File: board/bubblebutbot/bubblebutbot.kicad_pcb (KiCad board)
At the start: 2 copper layers, 94 x 32.5 mm, 55 parts, among them J1 JST XH, J10 JST XH, J11 JST XH, J13 JST XH, J2 USB_C_Receptacle, J3 Conn_01x03_Socket, J4 Conn_01x03_Socket, J5 Conn_01x03_Socket, J6 Conn_01x03_Socket, J7 Conn_01x03_Socket, J8 Conn_01x03_Socket, J9 JST XH, Q1 FDN336P, SW1 SW_Push, SW2 SW_Push, U1 DRV8833PWP, U2 ESP32-S3-WROOM-1, U3 AP2112K-3.3, U4 LIS3DH

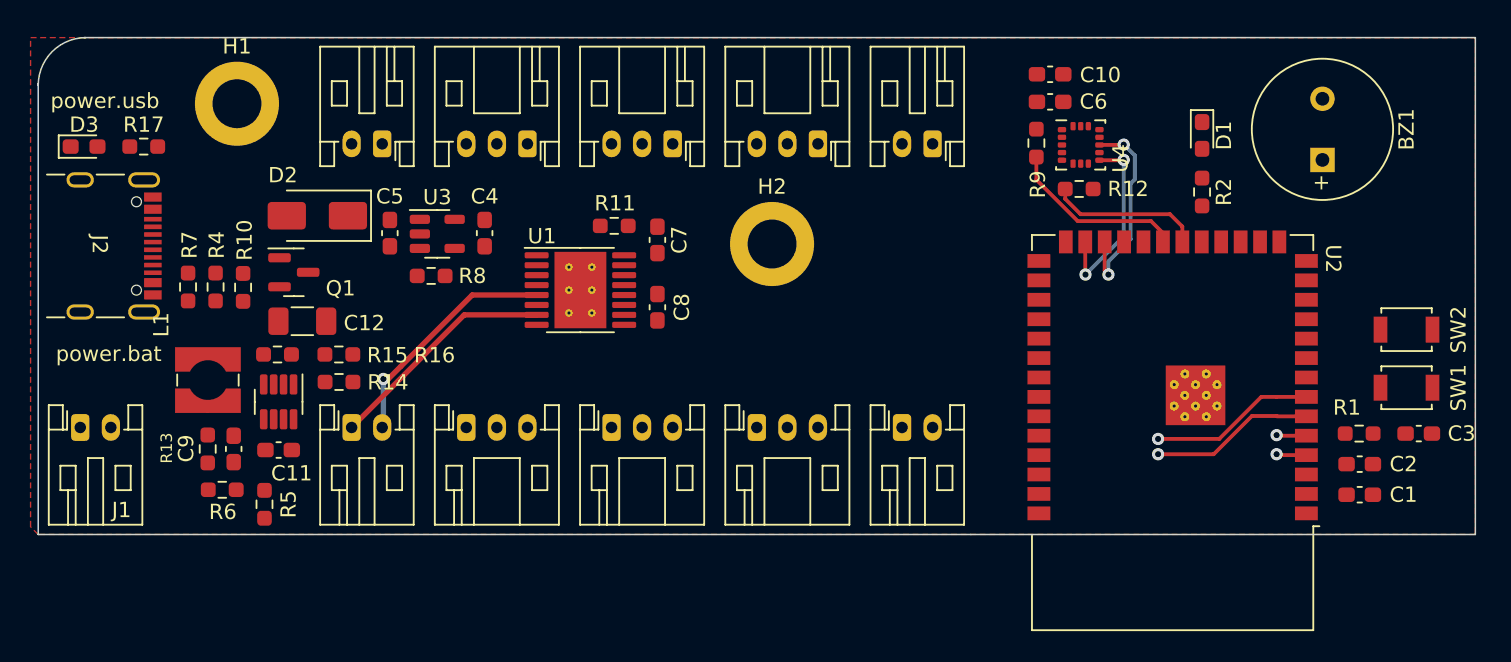
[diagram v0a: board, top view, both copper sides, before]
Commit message: pcb done!
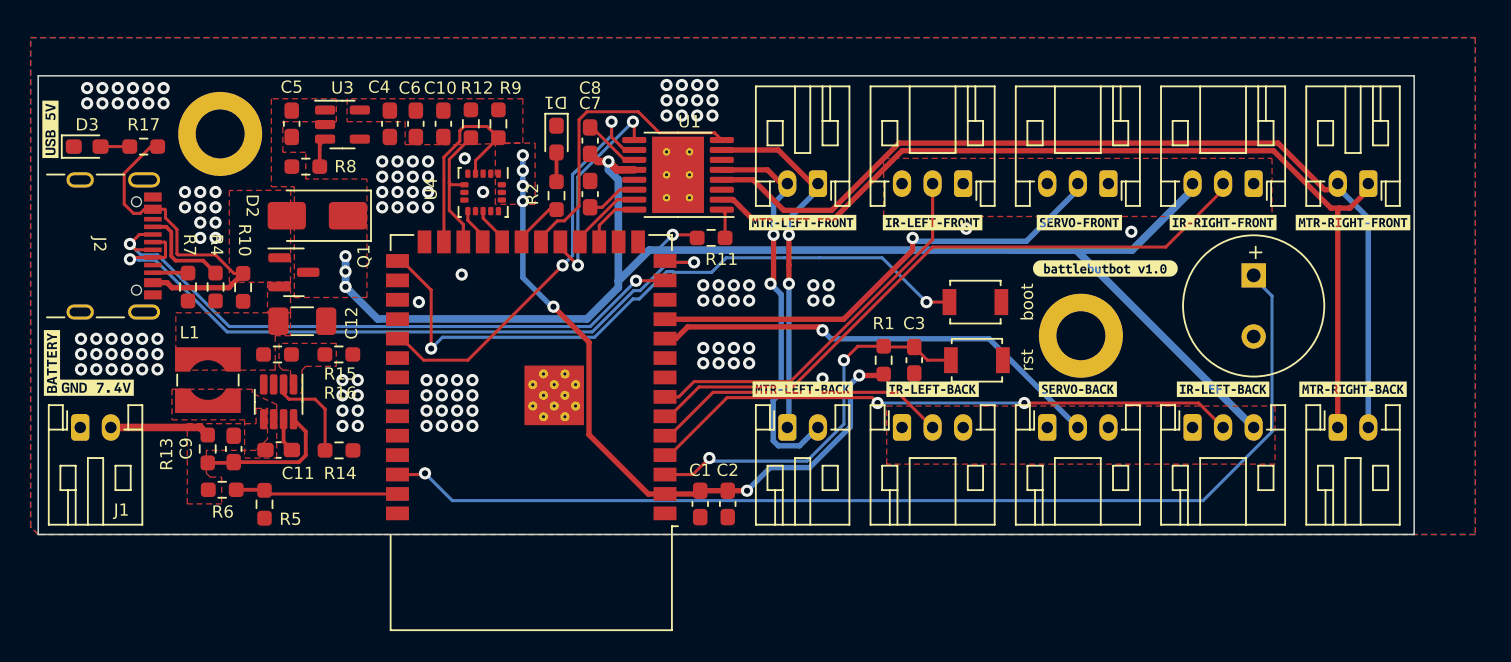
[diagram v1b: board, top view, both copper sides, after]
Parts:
- added kibuzzard-6507374A: G***, kibuzzard-6507374A, F.Cu at (115.5, 33.6)
- added kibuzzard-6507377B: G***, kibuzzard-6507377B, F.Cu at (124.0, 33.6)
- added kibuzzard-65073792: G***, kibuzzard-65073792, F.Cu at (133.6, 33.6)
- added kibuzzard-650737FA: G***, kibuzzard-650737FA, F.Cu at (143.0, 33.6)
- added kibuzzard-65073803: G***, kibuzzard-65073803, F.Cu at (151.5, 33.6)
- added kibuzzard-65073819: G***, kibuzzard-65073819, F.Cu at (115.5, 44.5)
- added kibuzzard-6507382A: G***, kibuzzard-6507382A, F.Cu at (124.0, 44.5)
- added kibuzzard-6507384E: G***, kibuzzard-6507384E, F.Cu at (133.5, 44.5)
- added kibuzzard-6507385B: G***, kibuzzard-6507385B, F.Cu at (143.0, 44.5)
- added kibuzzard-65073881: G***, kibuzzard-65073881, F.Cu at (151.5, 44.5)
- added kibuzzard-650738AB: G***, kibuzzard-650738AB, F.Cu at (135.3, 36.6)
- added kibuzzard-650739D2: G***, kibuzzard-650739D2, F.Cu at (69.3, 44.4)
- added kibuzzard-650739DD: G***, kibuzzard-650739DD, F.Cu at (66.4, 42.8)
- added kibuzzard-650739F6: G***, kibuzzard-650739F6, F.Cu at (66.3, 27.5)
- moved C1 43.1 mm to (108.8, 52.0), turned to -90 degrees
- moved D1 42.2 mm to (99.4, 28.1)
- moved R2 42.2 mm to (99.4, 31.8)
- moved U2 41.9 mm to (97.8, 47.4)
- moved C6 41.5 mm to (90.2, 27.1), turned to -90 degrees
- moved C2 41.4 mm to (110.6, 52.0), turned to -90 degrees
- moved R12 40.0 mm to (93.8, 27.1), turned to 90 degrees
- moved C10 39.8 mm to (92.0, 27.1), turned to -90 degrees
- moved U4 39.2 mm to (94.6, 31.6), turned to -90 degrees
- moved R9 35.2 mm to (95.6, 27.1)
- moved C3 33.3 mm to (122.8, 42.6), turned to -90 degrees
- moved R1 31.5 mm to (120.8, 42.6), turned to 90 degrees
- moved J10 28.6 mm to (116.5, 31.1)
- moved J13 28.6 mm to (152.5, 31.1)
- moved J3 28.6 mm to (126.0, 31.1)
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- renumbered SW2 to boot, SW1 to rst
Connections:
- C8 pad 2: 5V_SUPPLY -> +5V
- R11 pad 1: 5V_SUPPLY -> +5V
- U1 pad 12: 5V_SUPPLY -> +5V
- U2 pad 10: ESP32-MOTOR-AIN1 -> ESP32-SRV-B
- U2 pad 11: ESP32-MOTOR-AIN2 -> ESP32-SRV-F
- U2 pad 17: ESP32-SRV-B -> ESP32-MOTOR-AIN1
- U2 pad 18: ESP32-SRV-F -> ESP32-MOTOR-AIN2
- U2 pad 19: ESP32-OP-LED -> ESP32-MOTOR-BIN1
- U2 pad 20: ESP32-ACC-SDA -> ESP32-MOTOR-FAULT
- U2 pad 21: ESP32-ACC-SCL -> ESP32-OP-LED
- U2 pad 22: ESP32-MOTOR-FAULT -> ESP32-ACC-INT1
- U2 pad 23: ESP32-MOTOR-BIN1 -> ESP32-ACC-INT2
- U2 pad 24: ESP32-ACC-INT1 -> ESP32-ACC-SDA
- U2 pad 25: ESP32-ACC-INT2 -> ESP32-ACC-SCL
- U2 pad 4: ESP32-IR-FL -> ESP32-IR-BR
- U2 pad 5: ESP32-IR-FR -> ESP32-IR-BL
- U2 pad 6: ESP32-IR-BL -> ESP32-IR-FR
- U2 pad 7: ESP32-IR-BR -> ESP32-IR-FL
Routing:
- net +5V: track 0.00 -> 97.7 mm, vias 0 -> 5
- net ESP32-BUZZER: track 0.00 -> 70.4 mm, vias 0 -> 1
- net MOTOR-RIGHT-BL: track 0.00 -> 61.0 mm
- net MOTOR-RIGHT-BR: track 0.00 -> 60.7 mm
- net ESP32-D+: track 0.00 -> 46.8 mm, vias 0 -> 2
- net +3.3V: track 0.00 -> 45.9 mm, vias 0 -> 7
- net ESP32-BOOT0: track 0.00 -> 44.4 mm, vias 0 -> 2
- net ESP32-D-: track 0.00 -> 41.9 mm, vias 0 -> 2
- net ESP32-IR-FR: track 1.97 -> 42.6 mm, vias 1 -> 0
- net ESP32-SRV-F: track 0.00 -> 31.2 mm, vias 0 -> 1
- net ESP32-SRV-B: track 0.00 -> 30.0 mm, vias 0 -> 1
- net ESP32-IR-BR: track 10.8 -> 38.9 mm, vias 1 -> 2
- net ESP32-MOTOR-BIN2: track 0.00 -> 27.5 mm, vias 0 -> 2
- net ESP32-RESET: track 0.00 -> 25.1 mm, vias 0 -> 2
- net ESP32-IR-FL: track 1.97 -> 25.0 mm, vias 1 -> 0
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- added copper zone on F.Cu, net +3.3V
- added copper zone on F.Cu, net +5V
- added copper zone on F.Cu, net +7.5V
- added copper zone on F.Cu, net 5V_BAT
- added copper zone on F.Cu, net 5V_USB_POWER
- added copper zone on B.Cu, net GND
- added copper zone on F.Cu, net Net-(U5-FB)
- added copper zone on F.Cu, net Net-(U5-LX)
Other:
- board size 94 x 32.5 mm -> 90 x 30 mm
- board text removed: "power.bat"
- board text removed: "power.usb"
